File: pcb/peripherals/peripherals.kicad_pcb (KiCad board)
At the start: 2 copper layers, 133.3 x 62.7 mm, 27 parts, among them J1 JST XH, J10 JST XH, J11 JST XH, J2 JST XH, J3 Pin header, J4 Pin header, J9 JST XH, Q1 IRFZ44N, Q2 IRFZ44N, U1 DFPlayer_Mini, U2 buck-converter

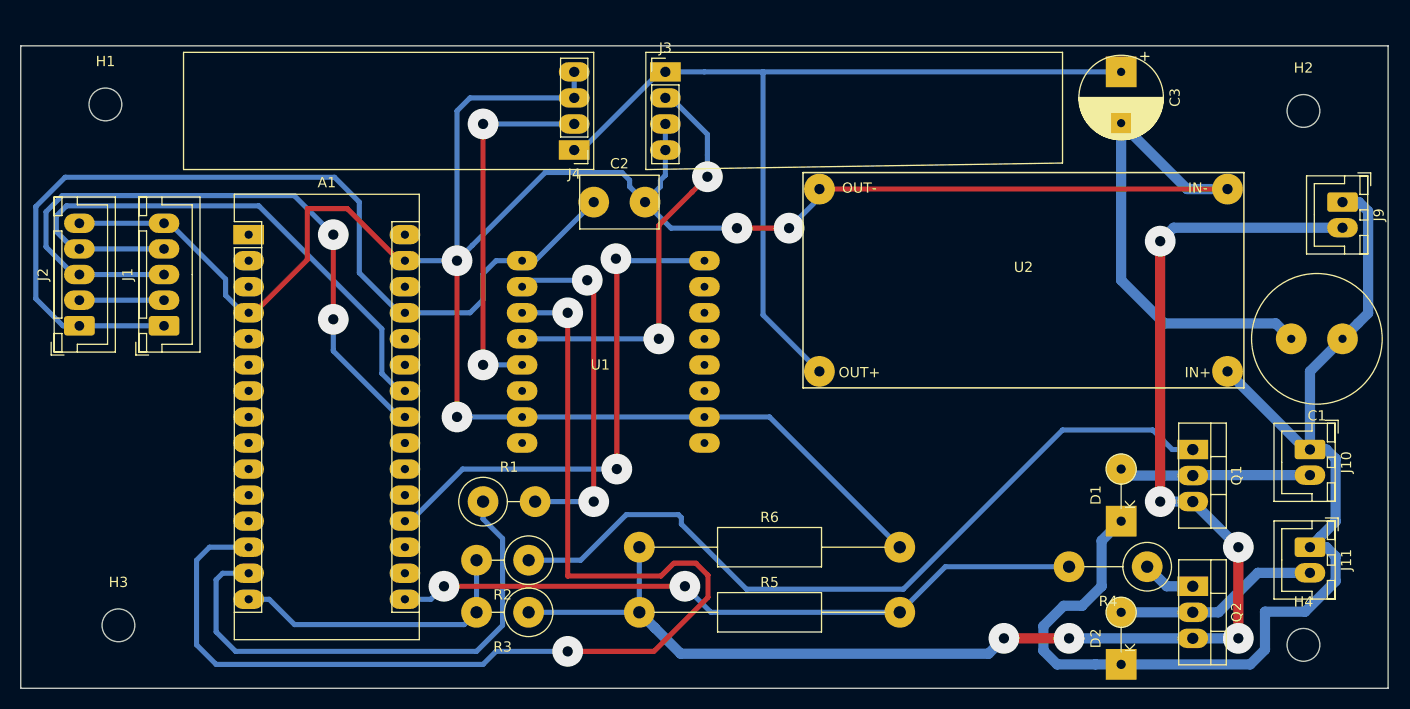
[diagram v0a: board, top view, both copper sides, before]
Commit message: SMD version.
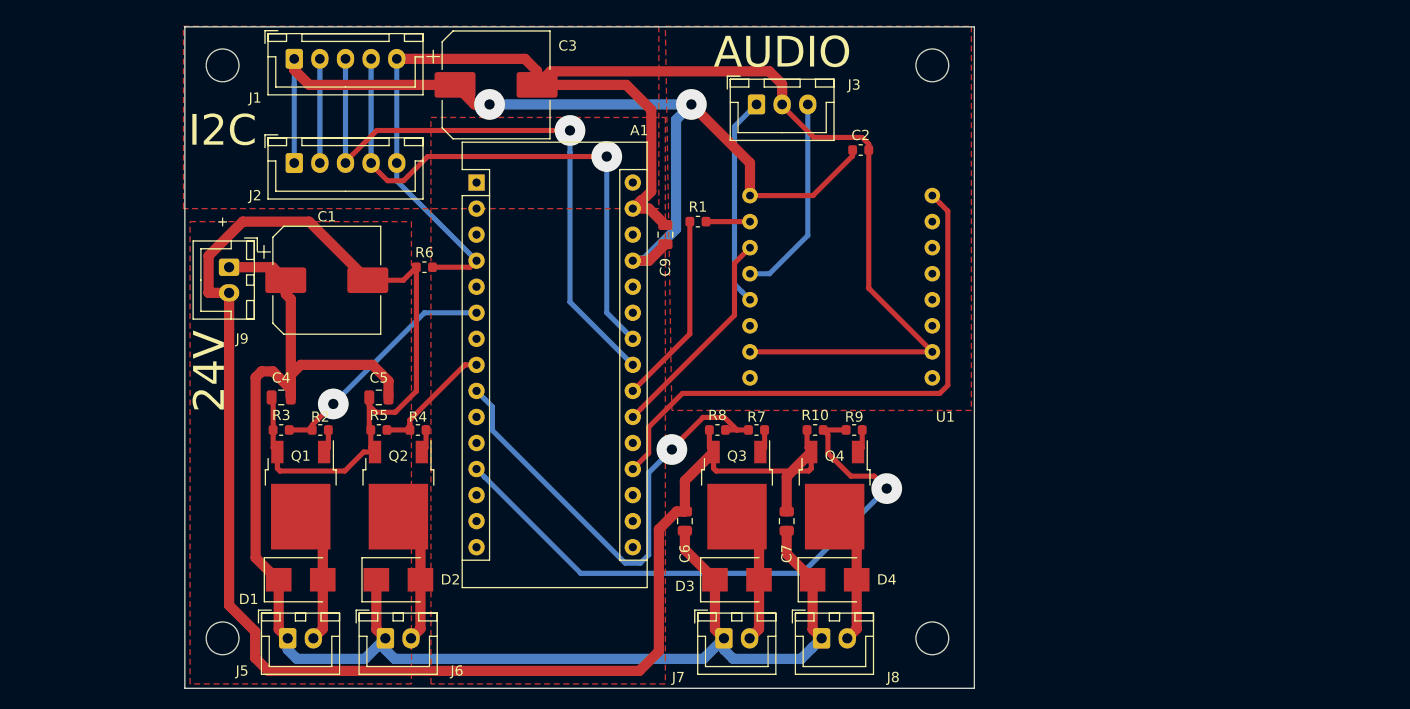
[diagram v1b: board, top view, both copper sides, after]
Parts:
- removed J10, J11: JST XH, Connector_JST:JST_XH_B02B-XH-A_1x02_P2.50mm_Vertical
- removed J4: Pin header, Connector_PinHeader_2.54mm:PinHeader_1x04_P2.54mm_Vertical
- removed U2: buck-converter, Peripherals:buck-converter
- added C4: 1u, Capacitor_SMD:C_0805_2012Metric, F.Cu at (25.4, 64.1)
- added C5: 1u, Capacitor_SMD:C_0805_2012Metric, F.Cu at (34.9, 64.1)
- added C6: 1u, Capacitor_SMD:C_0805_2012Metric, F.Cu at (64.8, 76.2)
- added C7: 1u, Capacitor_SMD:C_0805_2012Metric, F.Cu at (74.7, 76.2)
- added C9: 1u, Capacitor_SMD:C_0805_2012Metric, F.Cu at (62.9, 48.3)
- added D3: SS34, Diode_SMD:D_SMB, F.Cu at (69.8, 81.9)
- added D4: SS34, Diode_SMD:D_SMB, F.Cu at (79.4, 81.9)
- added J5: JST XH, Connector_JST:JST_XH_B02B-XH-A_1x02_P2.50mm_Vertical, F.Cu at (26.0, 87.6)
- added J6: JST XH, Connector_JST:JST_XH_B02B-XH-A_1x02_P2.50mm_Vertical, F.Cu at (35.6, 87.6)
- added J7: JST XH, Connector_JST:JST_XH_B02B-XH-A_1x02_P2.50mm_Vertical, F.Cu at (68.6, 87.6)
- added J8: JST XH, Connector_JST:JST_XH_B02B-XH-A_1x02_P2.50mm_Vertical, F.Cu at (78.1, 87.6)
- added Q3: FDD8447L, Package_TO_SOT_SMD:TO-252-2, F.Cu at (69.8, 73.7)
- added Q4: FDD8447L, Package_TO_SOT_SMD:TO-252-2, F.Cu at (79.4, 73.7)
- added R10: 47k, Resistor_SMD:R_0603_1608Metric, F.Cu at (77.5, 67.3)
- added R7: 1k, Resistor_SMD:R_0603_1608Metric, F.Cu at (71.8, 67.3)
- added R8: 47k, Resistor_SMD:R_0603_1608Metric, F.Cu at (67.9, 67.3)
- added R9: 1k, Resistor_SMD:R_0603_1608Metric, F.Cu at (81.3, 67.3)
- C1: footprint Capacitor_THT:C_Radial_D12.5mm_H20.0mm_P5.00mm -> Capacitor_SMD:CP_Elec_10x10
- C2: value 100n -> 1u; footprint Capacitor_THT:C_Disc_D7.5mm_W5.0mm_P5.00mm -> Capacitor_SMD:C_0603_1608Metric
- C3: footprint Capacitor_THT:CP_Radial_D8.0mm_P5.00mm -> Capacitor_SMD:CP_Elec_10x10
- D1, D2: value 1N4001 -> SS34; footprint Diode_THT:D_A-405_P5.08mm_Vertical_KathodeUp -> Diode_SMD:D_SMB
- J3: value Pin header -> Conn_01x03; footprint Connector_PinHeader_2.54mm:PinHeader_1x04_P2.54mm_Vertical -> Connector_JST:JST_XH_B03B-XH-A_1x03_P2.50mm_Vertical
- Q1, Q2: value IRFZ44N -> FDD8447L; footprint Package_TO_SOT_THT:TO-220-3_Vertical -> Package_TO_SOT_SMD:TO-252-2
- R1, R2, R3: footprint Resistor_THT:R_Axial_DIN0414_L11.9mm_D4.5mm_P5.08mm_Vertical -> Resistor_SMD:R_0603_1608Metric
- R4: footprint Resistor_THT:R_Axial_DIN0414_L11.9mm_D4.5mm_P7.62mm_Vertical -> Resistor_SMD:R_0603_1608Metric
- R5, R6: footprint Resistor_THT:R_Axial_DIN0411_L9.9mm_D3.6mm_P25.40mm_Horizontal -> Resistor_SMD:R_0603_1608Metric
- moved H4 119.6 mm to (19.7, 31.8)
- moved H2 117.3 mm to (19.7, 87.6)
- moved J9 108.8 mm to (20.3, 51.4)
- moved C1 99.2 mm to (29.8, 52.7), turned to 0 degrees
- moved H3 96.3 mm to (88.9, 31.8)
- moved H1 96.0 mm to (88.9, 87.6)
- moved Q1 87.1 mm to (27.3, 73.7)
- moved D1 80.2 mm to (27.3, 81.9), turned to 0 degrees
- moved Q2 78.0 mm to (36.8, 73.7)
- moved R4 72.4 mm to (38.7, 67.3)
- moved D2 71.0 mm to (36.8, 81.9), turned to 0 degrees
- moved C3 61.0 mm to (46.4, 33.7), turned to 0 degrees
- moved R1 34.4 mm to (66.0, 47.0)
- moved R6 34.4 mm to (39.4, 51.4)
- moved R5 31.0 mm to (34.9, 67.3)
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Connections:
- A1 pad 12: Net-(A1-Pad12) -> PWM4
- A1 pad 15: PWM1 -> Net-(A1-Pad15)
- A1 pad 16: PWM2 -> Net-(A1-Pad16)
- A1 pad 21: Net-(A1-Pad21) -> DFTX
- A1 pad 22: Net-(A1-Pad22) -> DFRX
- A1 pad 6: Net-(A1-Pad6) -> PWM1
- A1 pad 8: Net-(A1-Pad8) -> PWM2
- A1 pad 9: Net-(A1-Pad9) -> PWM3
- C1 pad 2: GND -> GNDPWR
- C3 pad 1: +5VP -> +5V
- J3 pad 1: +5VP -> Net-(J3-Pad1)
- J3 pad 2: Net-(J3-Pad2) -> GND
- J3 pad 3: GND -> Net-(J3-Pad3)
- R1 pad 1: Net-(A1-Pad14) -> DFRX
- U1 pad 3: Net-(A1-Pad13) -> DFTX
- U1 pad 4: Net-(J3-Pad2) -> Net-(J3-Pad3)
- U1 pad 5: Net-(J4-Pad2) -> Net-(J3-Pad1)
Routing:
- net GND: track 282.5 -> 147.1 mm, vias 4 -> 0
- net Net-(A1-Pad13): track 114.2 -> 0.00 mm, vias 2 -> 0
- net +5VP: track 88.0 -> 0.00 mm
- net Net-(Q1-Pad1): track 77.2 -> 2.32 mm
- net PWM4: track 0.00 -> 59.5 mm, vias 0 -> 1
- net PWM2: track 68.2 -> 11.9 mm, vias 2 -> 0
- net GNDPWR: track 139.9 -> 195.9 mm, vias 6 -> 0
- net Net-(A1-Pad14): track 51.2 -> 0.00 mm
- net PWM3: track 0.00 -> 47.1 mm, vias 0 -> 1
- net +24V: track 108.9 -> 152.3 mm
- net Net-(J3-Pad2): track 40.8 -> 0.00 mm, vias 2 -> 0
- net Net-(J4-Pad2): track 36.2 -> 0.00 mm, vias 2 -> 0
- net Net-(R1-Pad2): track 34.2 -> 4.29 mm, vias 2 -> 0
- net DFTX: track 0.00 -> 21.2 mm
- net Net-(J3-Pad1): track 0.00 -> 20.6 mm
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- added copper zone on F.Cu, net GND
- added copper zone on F.Cu, net GNDPWR
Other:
- board size 133.3 x 62.7 mm -> 77 x 64.5 mm
- board text added: "+"
- board text added: "24V"
- board text added: "AUDIO"
- board text added: "I2C"
